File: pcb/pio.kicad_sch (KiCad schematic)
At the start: 50 parts, among them J11 BM04B-SRSS-TB, J4 BM06B-SRSS-TB, J5 BM06B-SRSS-TB, J6 BM04B-SRSS-TB, J7 BM06B-SRSS-TB, U4 MCP23017T-E/ML

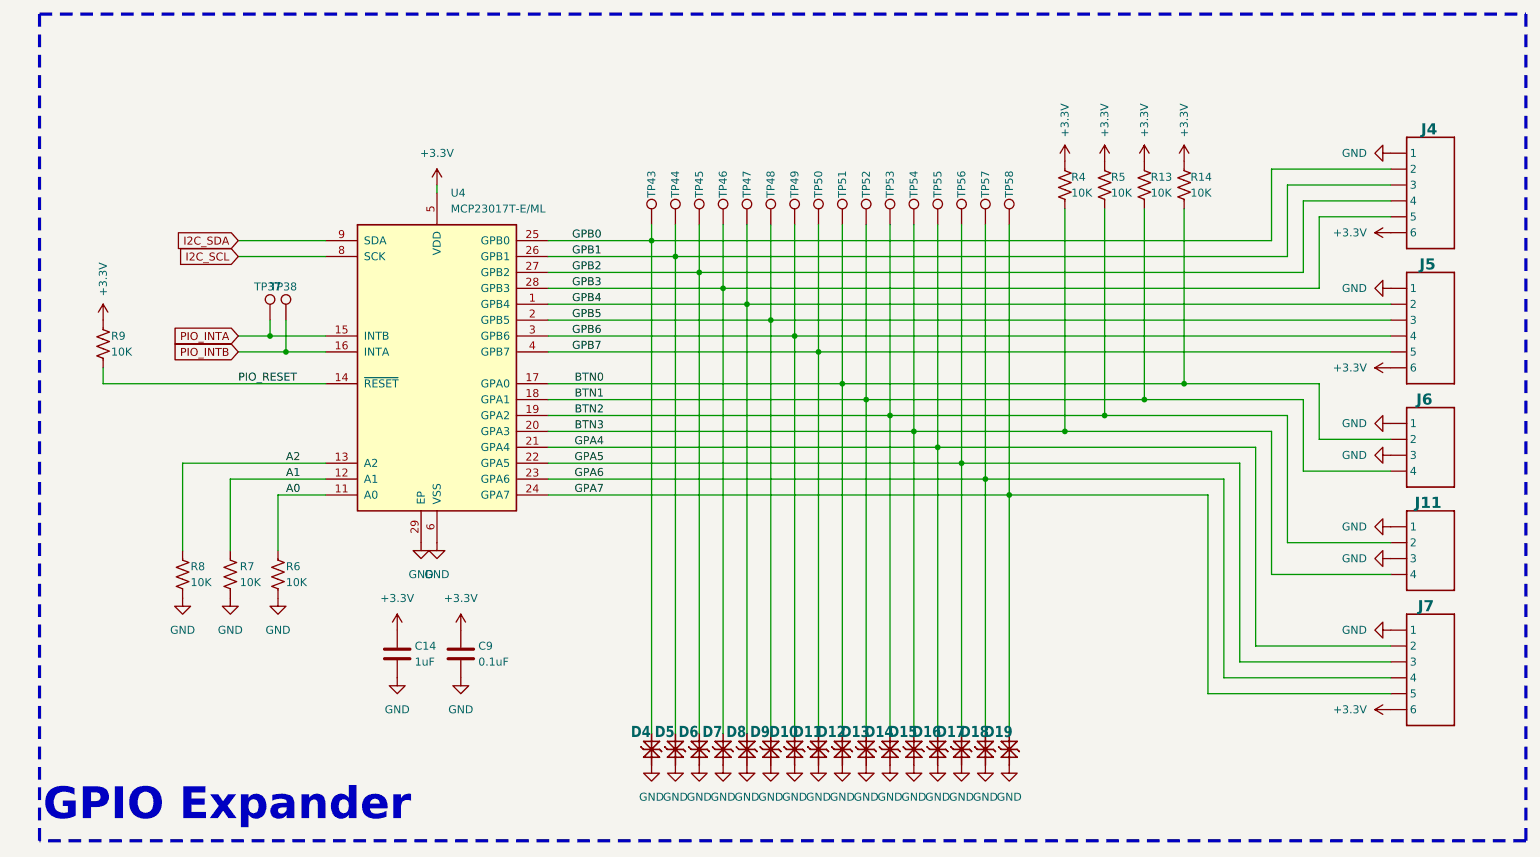
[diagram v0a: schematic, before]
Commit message: Clean up and consistency
Moved buzzer to MCU
Fixed model directory
Set font size
Set outline size
Upscaled Roxy ❤️
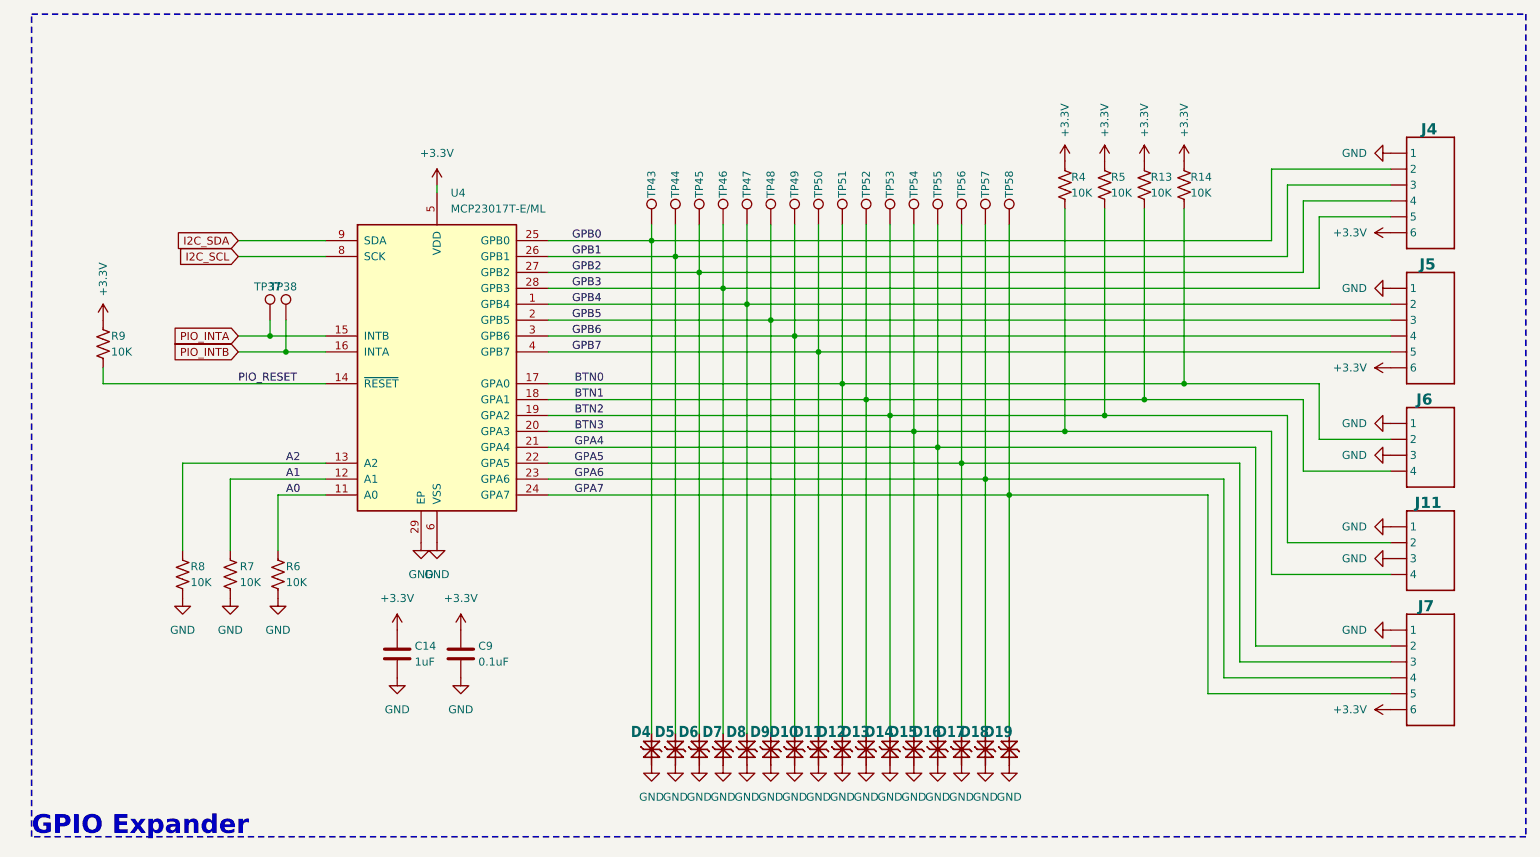
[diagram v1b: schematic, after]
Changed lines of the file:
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@@
 	)
 	(rectangle
-		(start 16.51 15.875)
-		(end 254 147.955)
+		(start 15.24 15.875)
+		(end 254 147.32)
 		(stroke
-			(width 0.508)
+			(width 0.254)
 			(type dash)
 			(color 255 153 0 1)
@@
 	(text "GPIO Expander"
 		(exclude_from_sim yes)
-		(at 46.482 142.24 0)
+		(at 15.24 147.32 0)
 		(effects
 			(font
 				(face "KiCad Font")
-				(size 5.08 5.08)
+				(size 3 3)
 				(thickness 1.016)
 				(bold yes)
-				(color 255 153 0 1)
+				(color 0 0 194 1)
 			)
+			(justify left bottom)
 		)
 	)
